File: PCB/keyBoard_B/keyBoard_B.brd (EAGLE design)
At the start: 169.5 x 134.6 mm, 281 parts

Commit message: fw
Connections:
- net BD1: now also J72.2, SV4.8; no longer J70.2, SV4.10
- net BD3: now also J70.2, SV4.10; no longer J72.2, SV4.8
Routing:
- net BD3: track 53.8 -> 44.2 mm
- net BD1: track 44.2 -> 53.8 mm
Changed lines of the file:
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@@
 <wire x1="161.99525" y1="142.875" x2="163.35375" y2="141.5165" width="0.6096" layer="16"/>
 </signal>
-<signal name="BD1">
+<signal name="BD3">
 <contactref element="SV4" pad="10"/>
 <contactref element="J70" pad="2"/>
@@
 <wire x1="93.345" y1="120.3325" x2="89.2175" y2="123.66625" width="0.6096" layer="16"/>
 </signal>
-<signal name="BD3">
+<signal name="BD1">
 <contactref element="SV4" pad="8"/>
 <contactref element="J72" pad="2"/>

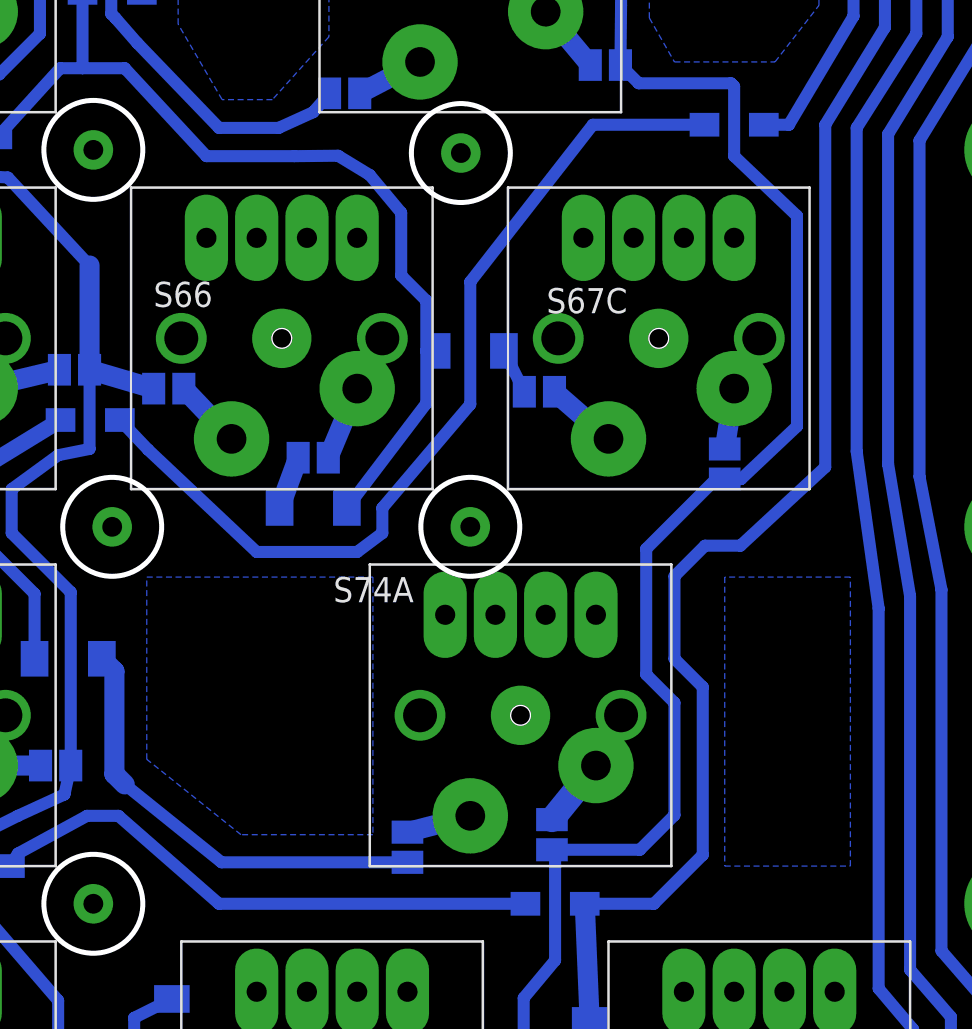
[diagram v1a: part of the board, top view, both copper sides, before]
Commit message: add1
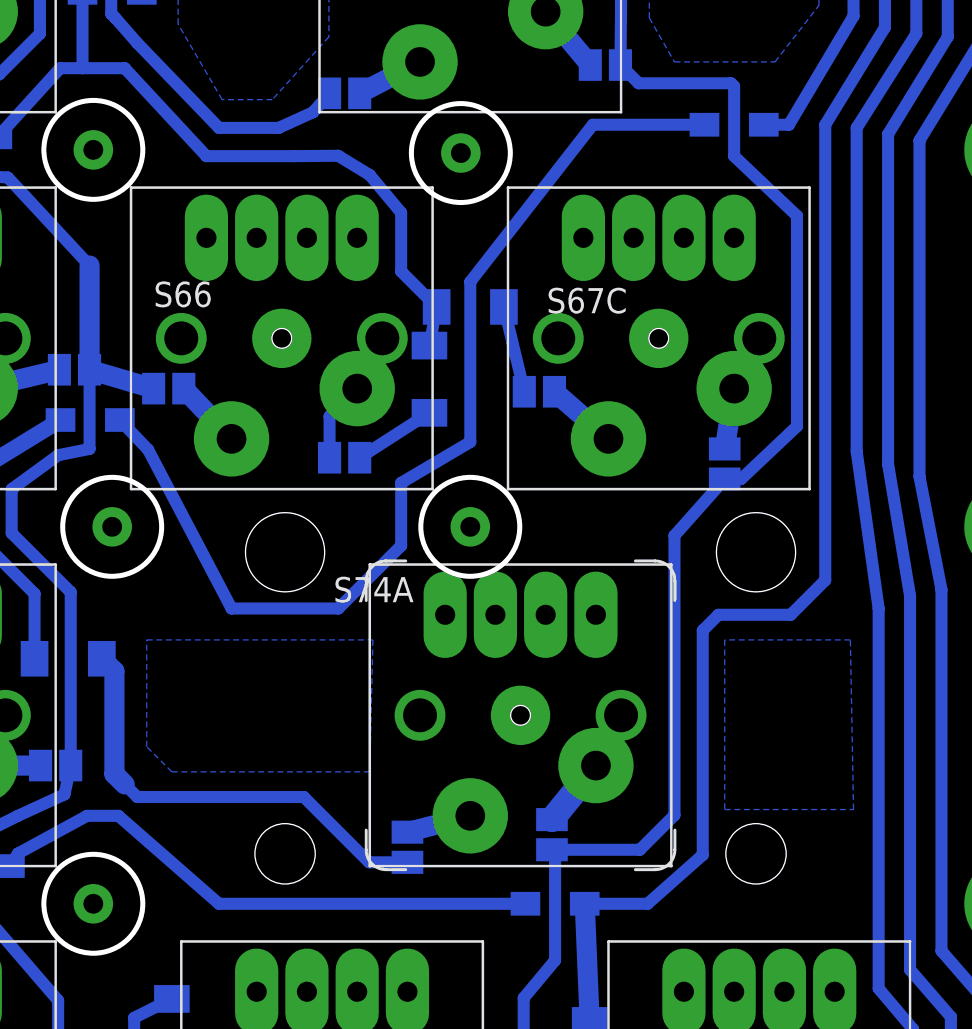
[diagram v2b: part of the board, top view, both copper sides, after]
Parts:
- added STAB_RSP: STAB, kbmxco:ZEALIOS-PCB_2U
- moved D68 8.77 mm to (162.2, 86.8), turned to 90 degrees
- moved D67B 2.22 mm to (164.3, 90.5)
- moved JB66 1.59 mm to (158.0, 82.9), turned to 0 degrees
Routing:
- net B3J: track 46.2 -> 36.8 mm
- net N$399: track 46.3 -> 52.1 mm
- net N$331: track 2.31 -> 4.41 mm
- net N$288: track 2.71 -> 4.19 mm
- net N$393: track 153.2 -> 152.1 mm
